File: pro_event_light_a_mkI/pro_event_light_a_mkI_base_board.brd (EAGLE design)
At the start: 107.7 x 88.4 mm, 93 parts, among them K1 62201021121, SW1 ALPS_EC11D

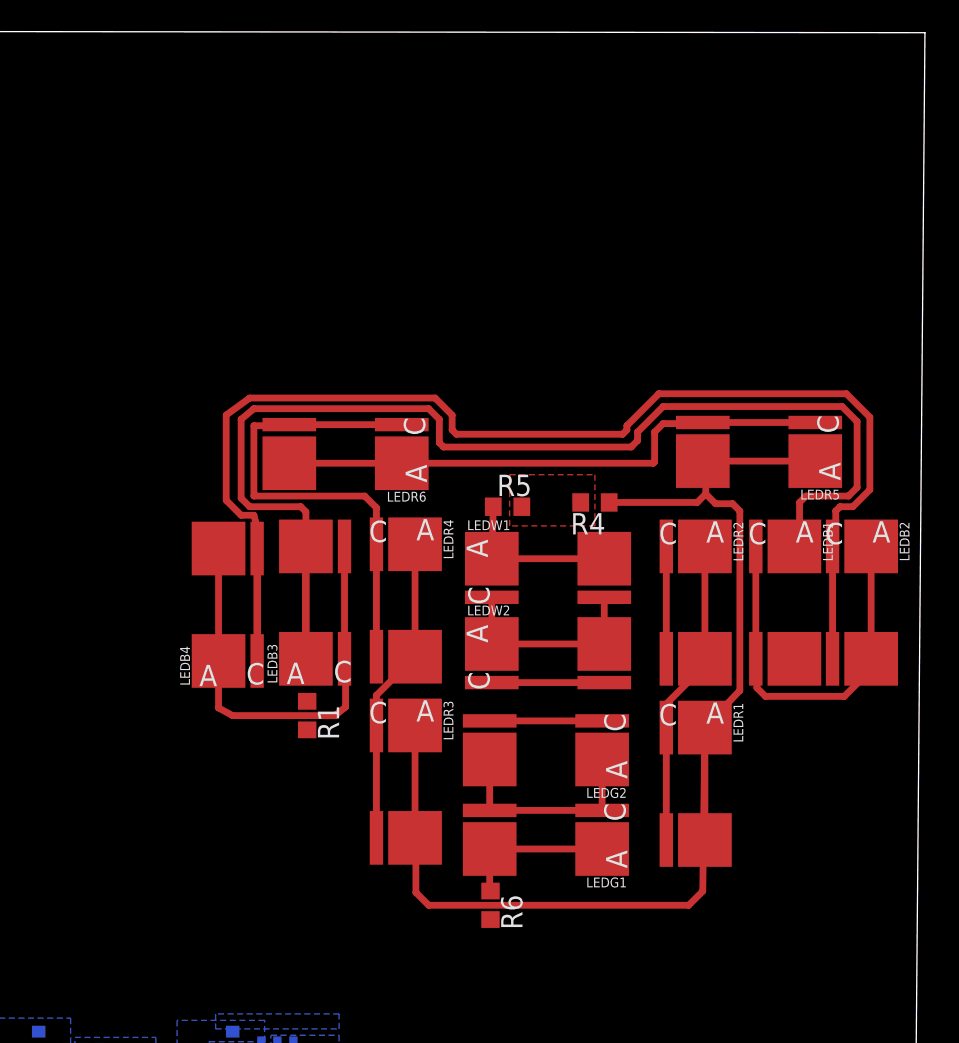
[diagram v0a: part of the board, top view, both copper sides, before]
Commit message: first push to remote repository
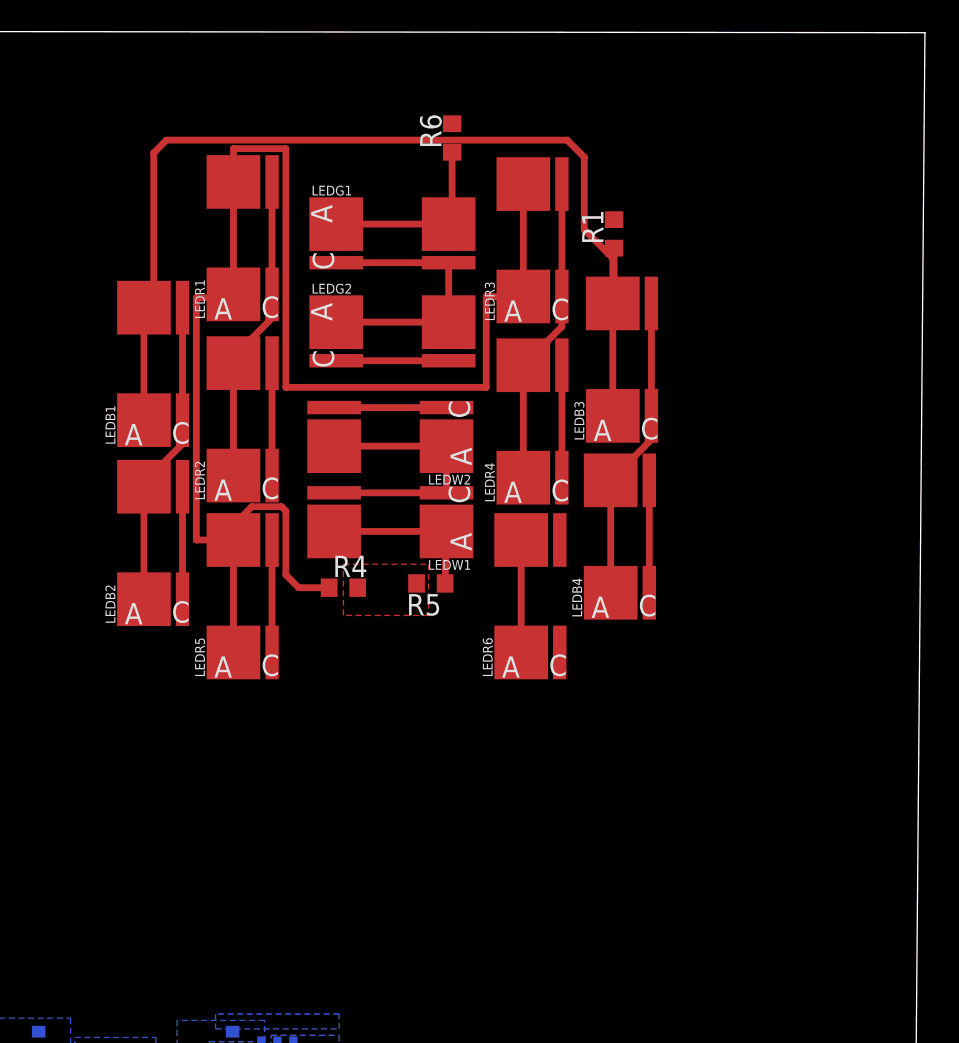
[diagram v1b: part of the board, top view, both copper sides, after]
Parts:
- moved R6 45.8 mm to (79.5, 81.9), turned to 90 degrees
- moved LEDR1 40.9 mm to (68.1, 75.9), turned to 90 degrees
- moved LEDB2 40.3 mm to (62.7, 57.8), turned to 90 degrees
- moved LEDB1 38.3 mm to (62.7, 68.5), turned to 90 degrees
- moved LEDG1 35.2 mm to (75.9, 75.2), turned to 0 degrees
- moved R1 34.0 mm to (89.2, 76.2), turned to 90 degrees
- moved LEDR3 33.7 mm to (85.3, 75.8), turned to 90 degrees
- moved LEDR5 31.2 mm to (68.1, 54.6), turned to 90 degrees
- moved LEDR2 27.2 mm to (68.1, 65.2), turned to 90 degrees
- moved LEDG2 24.6 mm to (75.9, 69.3), turned to 0 degrees
- moved LEDB4 23.7 mm to (90.6, 58.2)
- moved LEDB3 23.3 mm to (90.7, 68.7)
- moved LEDW2 17.7 mm to (75.8, 65.2), turned to 180 degrees
- moved R4 15.8 mm to (73.0, 55.1), turned to 0 degrees
- moved LEDR6 15.4 mm to (85.2, 54.6), turned to 90 degrees
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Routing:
- net DRIVER_LEDB: track 80.2 -> 13.4 mm
- net DRIVER_LEDR: track 36.5 -> 13.4 mm
- net N$14: track 33.4 -> 13.4 mm
- net VSENSE_LEDR: track 76.6 -> 90.6 mm
- net VSENSE_LEDB: track 75.2 -> 62.0 mm
- net N$6: track 29.6 -> 18.2 mm
- net N$4: track 24.8 -> 18.3 mm
- net N$3: track 12.8 -> 16.9 mm
- net N$25: track 12.3 -> 16.2 mm
- net VSENSE_LEDG: track 9.22 -> 11.1 mm
